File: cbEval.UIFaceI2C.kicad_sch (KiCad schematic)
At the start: 20 parts, among them J10 Bergstik-II_1x3, U1 MCP23017-E/SP, U2 MCP23017-E/SP, U3 ATtiny85-20PU

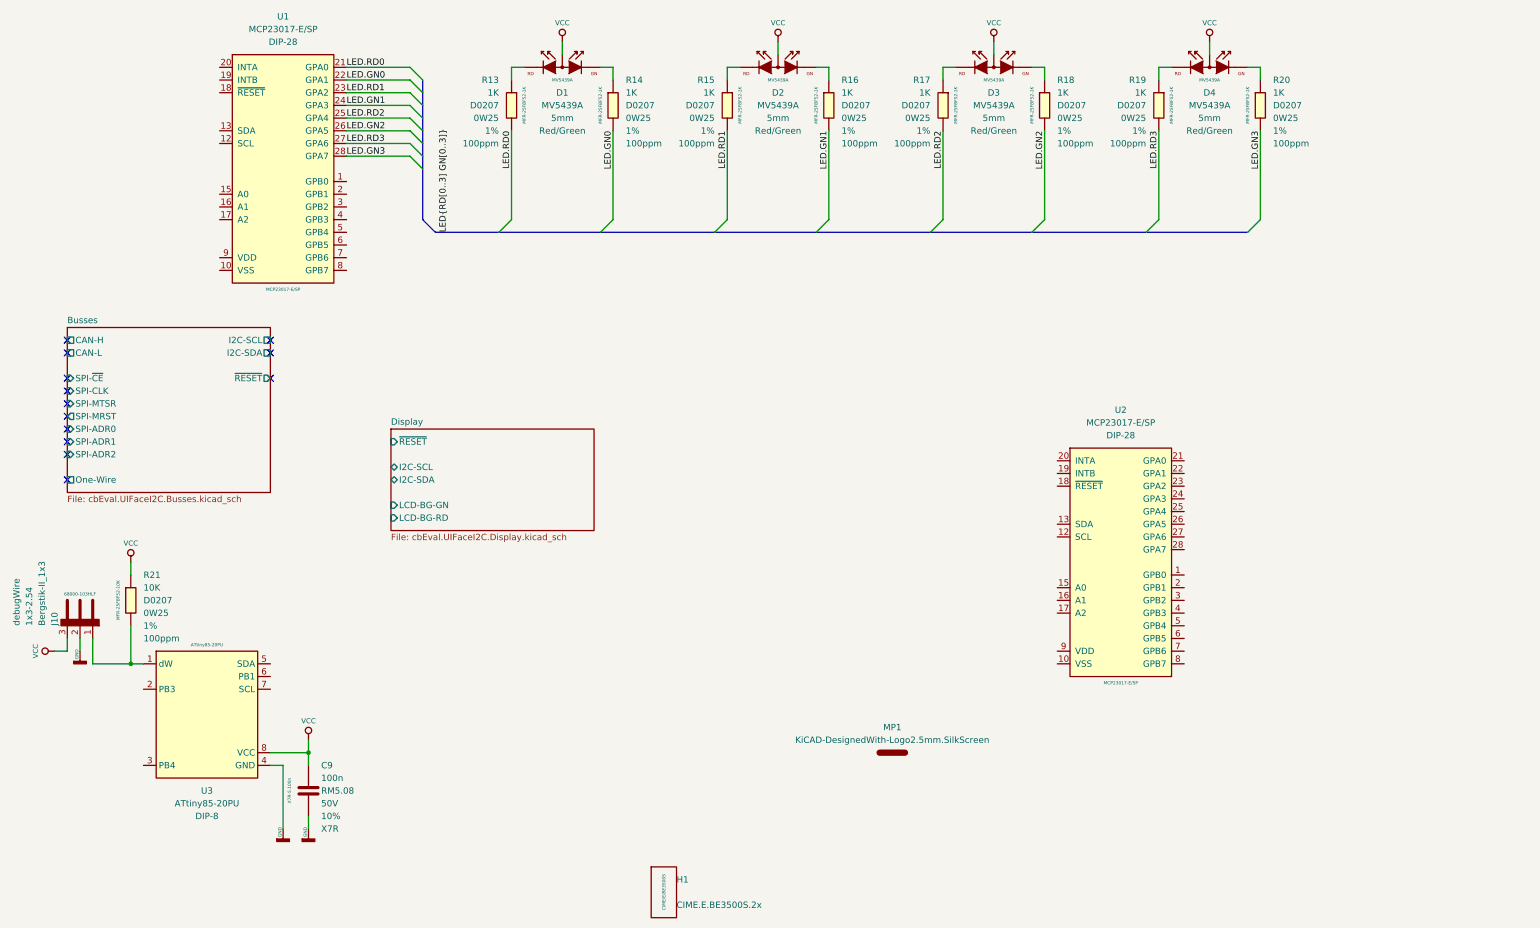
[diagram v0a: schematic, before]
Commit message: Bauteile aktualisiert
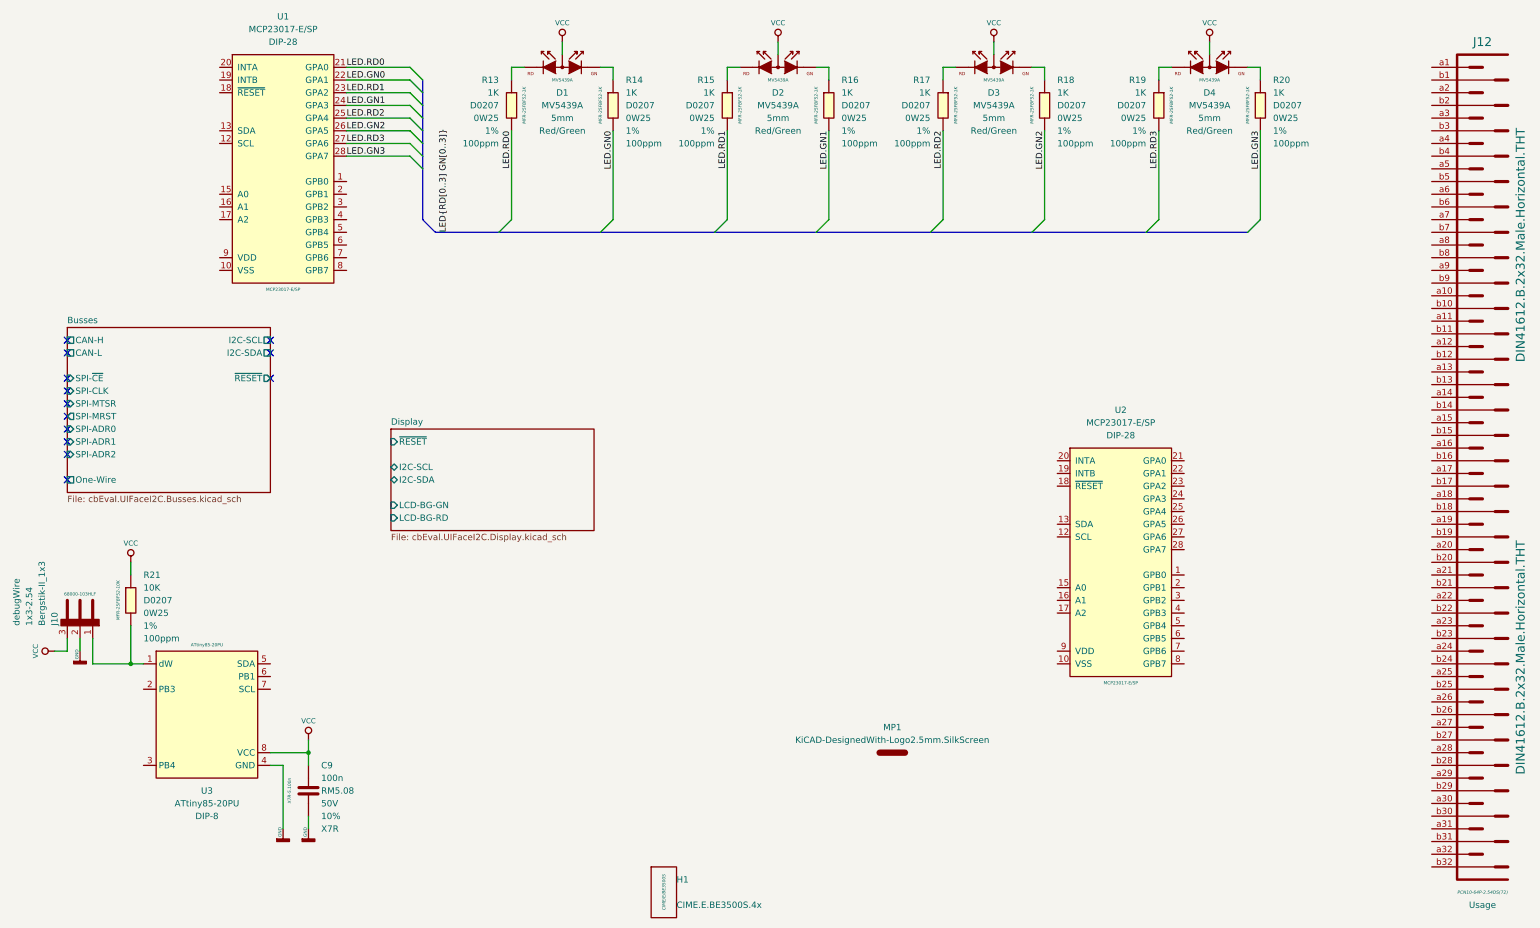
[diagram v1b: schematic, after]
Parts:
- added J12: DIN41612.B.2x32.Male.Horizontal.THT, BTech.Connector.DIN41612:DIN41612.B.2x32.Male.Horizontal.THT, symbol J.DIN41612:DIN41612.B.2x32.Male.Horizontal.THT
- C9: ID X7R-5.100n -> (none); MPN (none) -> X7R-5.100n
- D1, D2, D3, D4: ID MV5439A -> (none); MPN (none) -> MV5439A
- H1: value CIME.E.BE3500S.2x -> CIME.E.BE3500S.4x; ID CIME/E/BE3500S -> (none); MPN (none) -> CIME/E/BE3500S
- J10: ID 68000-103HLF -> (none); MPN (none) -> 68000-103HLF
- R13, R14, R15, R16, R17, R18, R19, R20: ID MFR-25FBF52-1K -> (none); MPN (none) -> MFR-25FBF52-1K
- R21: ID MFR-25FBF52-10K -> (none); MPN (none) -> MFR-25FBF52-10K
- U1, U2: ID MCP23017-E/SP -> (none); MPN (none) -> MCP23017-E/SP
- U3: ID ATtiny85-20PU -> (none); MPN (none) -> ATtiny85-20PU
